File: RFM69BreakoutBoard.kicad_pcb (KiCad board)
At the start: 2 copper layers, 25.7 x 25.4 mm, 16 parts, among them P1 CONN_7, U1 MCP1703, U2 74LVC2, U3 74AHC1G, U4 RFM69HW

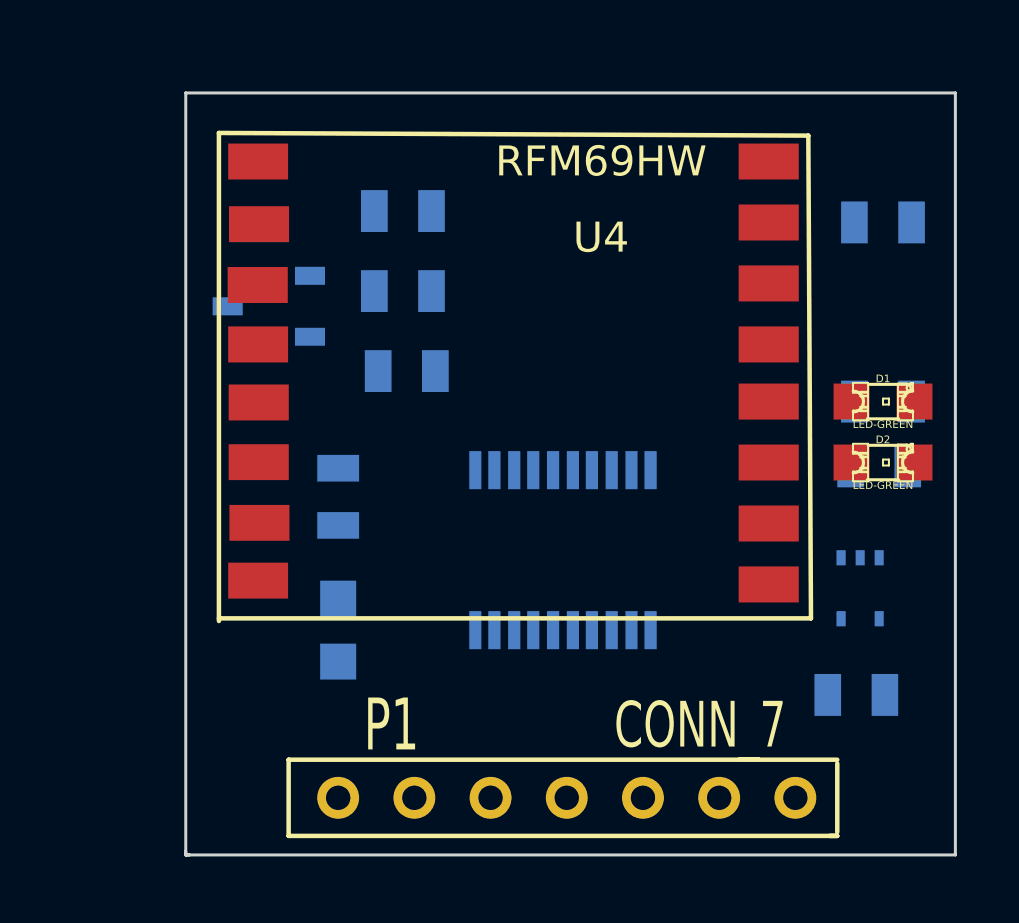
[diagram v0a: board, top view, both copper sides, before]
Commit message: clean up
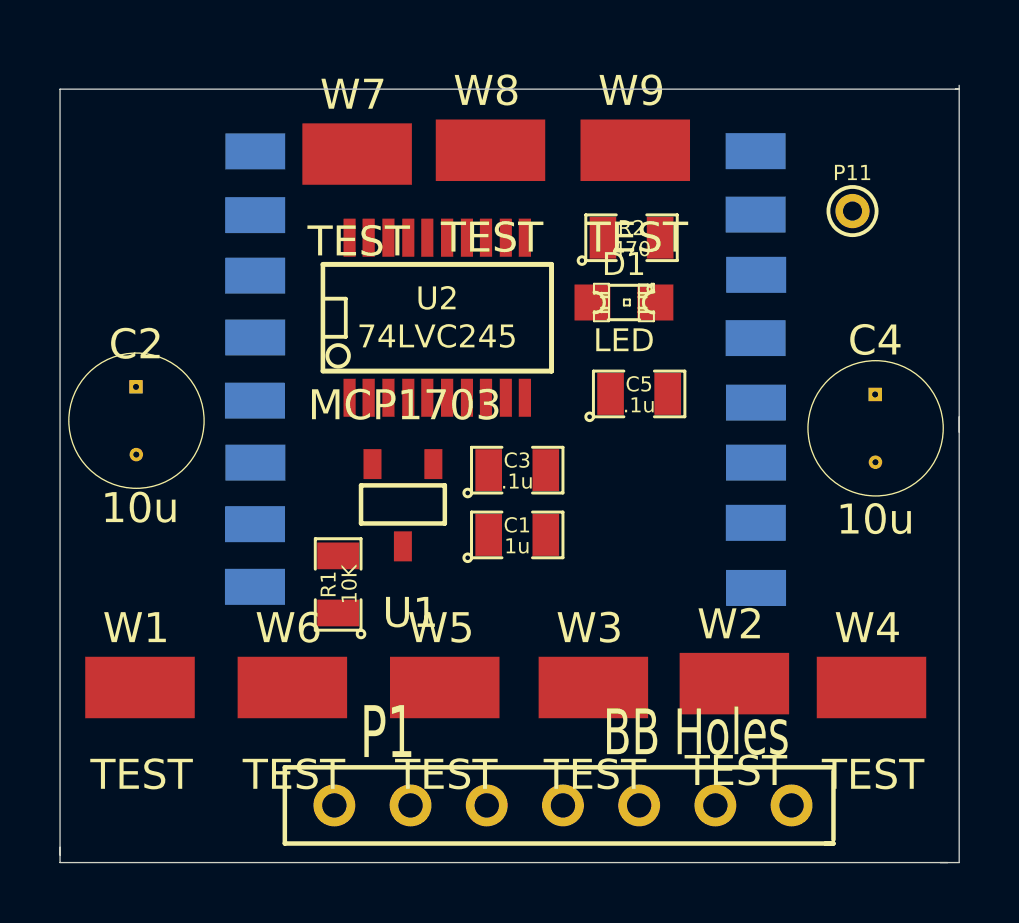
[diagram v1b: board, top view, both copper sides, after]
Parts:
- removed D2, D3: LED-GREEN, LED-0805
- removed R3, R4: 0, SM0805
- removed R5: 270, SM0805
- removed U4: RFM69HW, RFM69HW
- added C4: 10u, 10uCap, F.Cu at (107.4, 150.2)
- added C5: .1u, SM0805, F.Cu at (99.6, 149.1)
- added P11: ANA hole, PINTST, F.Cu at (106.7, 143.0)
- added W1: TEST, SMTST, F.Cu at (82.9, 158.9)
- added W2: TEST, SMTST, F.Cu at (102.7, 158.8)
- added W3: TEST, SMTST, F.Cu at (98.0, 158.9)
- added W4: TEST, SMTST, F.Cu at (107.3, 158.9)
- added W5: TEST, SMTST, F.Cu at (93.1, 158.9)
- added W6: TEST, SMTST, F.Cu at (88.0, 158.9)
- added W7: TEST, SMTST, F.Cu at (90.2, 141.1)
- added W8: TEST, SMTST, F.Cu at (94.6, 141.0)
- added W9: TEST, SMTST, F.Cu at (99.4, 141.0)
- C1, C3, U1: moved to F.Cu
- C2: footprint SM0805 -> 10uCap; moved to F.Cu
- D1: value LED-GREEN -> LED
- P1: value CONN_7 -> BB Holes
- R1: value 270 -> 10K; moved to F.Cu
- R2: value 270 -> 470; moved to F.Cu
- U2: value 74LVC2 -> 74LVC245; moved to F.Cu
- U3: value 74AHC1G -> RFM69HW; footprint SOT353 -> RFM69HW
- moved R1 19.2 mm to (89.5, 155.4), turned to 90 degrees
- moved U3 14.7 mm to (94.7, 147.3), turned to 0 degrees
- moved R2 11.2 mm to (99.3, 143.9), turned to 0 degrees
- moved C2 9.88 mm to (82.8, 150.0)
- moved C3 9.44 mm to (95.5, 151.6)
- moved D1 9.25 mm to (99.1, 146.1)
- moved U1 9.02 mm to (93.1, 152.1), turned to 180 degrees
- moved U2 8.81 mm to (92.8, 146.6), turned to 0 degrees
- moved C1 6.59 mm to (95.5, 153.8)
- moved P1 0.28 mm to (95.8, 162.8)
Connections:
- D1 pad 1: /MISO -> N-0000010
- D1 pad 2: /LED -> N-0000011
- P1 pad 1: /5V -> +5V
- P1 pad 3: /CLK -> /CLK_5V
- P1 pad 5: /MOSI -> /MOSI_5V
- P1 pad 6: /CS -> /CS_5V
- R1 pad 1: /LED -> /CS_5V
- R1 pad 2: GND -> +5V
- R2 pad 1: /LED -> N-0000011
- R2 pad 2: GND -> /CS_3V3
- U2 pad 1: (no net) -> +3.3V
- U2 pad 15: (no net) -> N-0000010
- U2 pad 16: /CS -> /CS_3V3
- U2 pad 17: /MOSI -> /MOSI_3V3
- U2 pad 18: /CLK -> /CLK_3V3
- U2 pad 2: /CLK -> N-000004
- U2 pad 3: /MOSI -> N-000007
- U2 pad 4: /CS -> N-000008
- U2 pad 5: (no net) -> N-000004
- U2 pad 6: (no net) -> GND
- U2 pad 7: (no net) -> GND
- U2 pad 8: (no net) -> GND
- U2 pad 9: (no net) -> GND
- U3 pad 1: /CS -> (no net)
- U3 pad 2: /MISO -> N-000001
- U3 pad 3: GND -> (no net)
- U3 pad 4: /MISO -> (no net)
- U3 pad 5: +3.3V -> (no net)
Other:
- board size 25.7 x 25.4 mm -> 30 x 25.9 mm
